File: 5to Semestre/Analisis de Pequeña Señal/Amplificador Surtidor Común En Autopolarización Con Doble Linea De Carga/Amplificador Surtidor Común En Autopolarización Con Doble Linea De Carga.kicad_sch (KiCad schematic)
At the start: 9 parts, among them Q1 NJFET

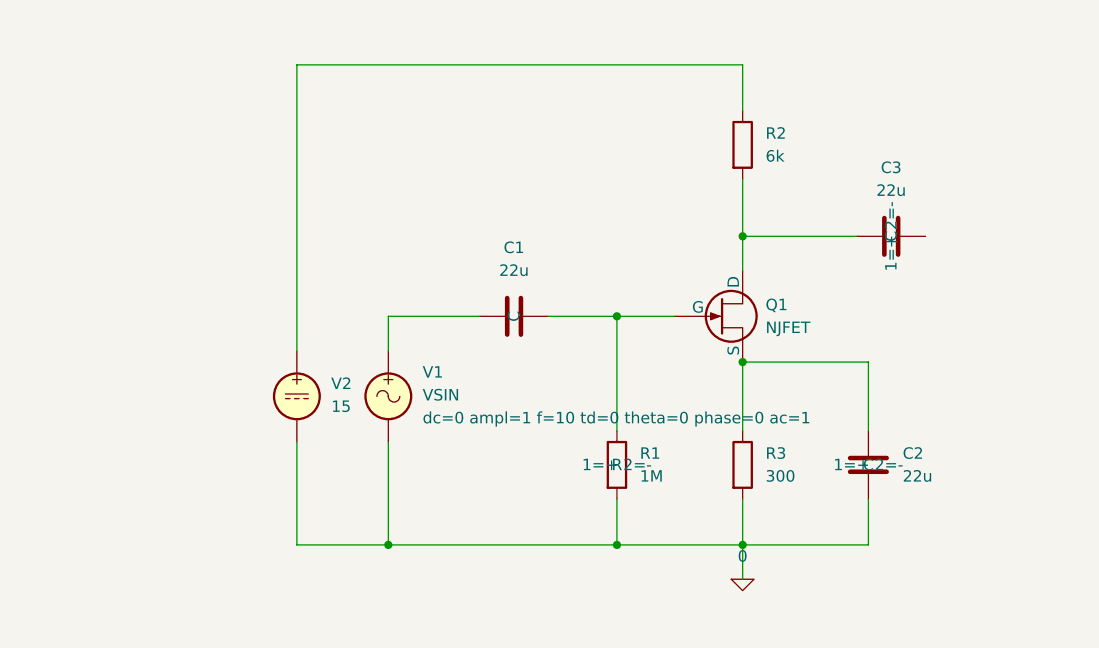
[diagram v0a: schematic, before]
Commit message: añadiendo Rc para simulaciones con carga y uso de etiquetas
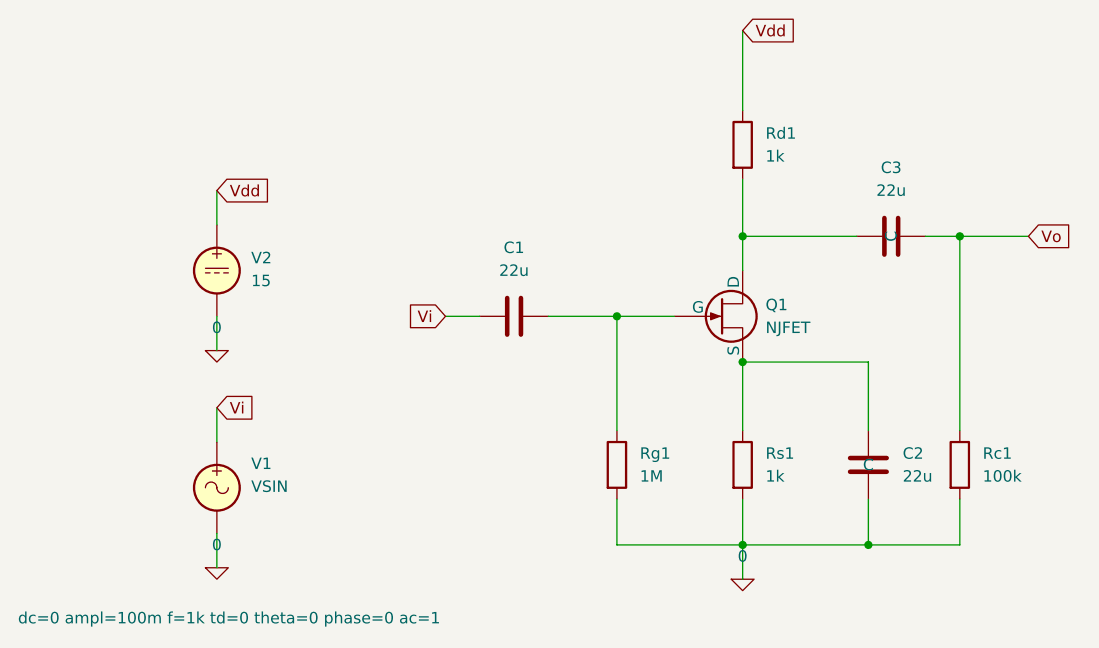
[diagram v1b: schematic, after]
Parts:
- added Rc1: 100k, symbol Device:R
- Rd1: renamed from R2; value 6k -> 1k
- Rs1: renamed from R3; value 300 -> 1k
- renumbered R1 to Rg1
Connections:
- net 0: now also Rc1.2
- net Vdd: now reaches Rd1.1, V2.1
- net Vo: now reaches C3.2
- net Vo: now also Rc1.1
- net Vi: now reaches C1.1, V1.1
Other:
- moved on the sheet: V1, V2
